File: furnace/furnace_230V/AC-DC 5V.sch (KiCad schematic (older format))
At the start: 14 parts

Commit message: Add files via upload
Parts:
- L?: value L_Core_Iron_Coupled_1243 -> PLA10AN3630R3D2
- PS?: value AC-DC 5V 700mA -> WX-DC12003 5V 0,7A
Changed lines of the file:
@@
 P 5900 4100
 F 0 "PS?" H 5900 4425 50  0000 C CNN
-F 1 "AC-DC 5V 700mA" H 5900 4334 50  0000 C CNN
+F 1 "WX-DC12003 5V 0,7A" H 5900 4334 50  0000 C CNN
 F 2 "" H 5900 3800 50  0001 C CNN
 F 3 "" H 6300 3750 50  0001 C CNN
@@
 P 4050 4100
 F 0 "L?" H 4050 4381 50  0000 C CNN
-F 1 "L_Core_Iron_Coupled_1243" H 4050 4290 50  0000 C CNN
+F 1 "PLA10AN3630R3D2" H 4050 4290 50  0000 C CNN
 F 2 "" H 4050 4100 50  0001 C CNN
 F 3 "~" H 4050 4100 50  0001 C CNN

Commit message: Add files via upload
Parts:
- C1, C2: renamed from C?; footprint (none) -> Capacitor_THT:C_Rect_L18.0mm_W7.0mm_P15.00mm_FKS3_FKP3; symbol Device:C -> furnace_230V-rescue:C-Device
- C3, C4: renamed from C?; footprint (none) -> Capacitor_SMD:C_1206_3216Metric_Pad1.33x1.80mm_HandSolder; symbol Device:C -> furnace_230V-rescue:C-Device
- C5: renamed from C?; footprint (none) -> Capacitor_SMD:C_Elec_5x5.4; symbol Device:CP -> furnace_230V-rescue:CP-Device
- D1: renamed from D?; footprint (none) -> Diode_SMD:D_SMA-SMB_Universal_Handsoldering; symbol Device:D_TVS -> furnace_230V-rescue:D_TVS-Device
- D2: renamed from D?; footprint (none) -> LED_SMD:LED_1206_3216Metric_Pad1.42x1.75mm_HandSolder; symbol Device:LED -> furnace_230V-rescue:LED-Device
- F1: renamed from F?; footprint (none) -> Fuse:Fuseholder_Cylinder-5x20mm_Stelvio-Kontek_PTF78_Horizontal_Open; symbol Device:Fuse -> furnace_230V-rescue:Fuse-Device
- L1: renamed from L?; symbol Device:L_Core_Iron_Coupled_1243 -> furnace_230V-rescue:L_Core_Iron_Coupled_1243-Device
- L2: renamed from L?; symbol Device:L -> furnace_230V-rescue:L-Device
- R1: renamed from R?; symbol Device:R -> furnace_230V-rescue:R-Device
- TP1, TP2: renamed from TP?; symbol Connector:TestPoint -> furnace_230V-rescue:TestPoint-Connector
- gave numbers to parts that had none: 1
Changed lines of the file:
@@
 $EndDescr
 $Comp
-L ac-dc:AC-DC PS?
+L ac-dc:AC-DC PS1
 U 1 1 60AB52E3
 P 5900 4100
-F 0 "PS?" H 5900 4425 50  0000 C CNN
+F 0 "PS1" H 5900 4425 50  0000 C CNN
 F 1 "WX-DC12003 5V 0,7A" H 5900 4334 50  0000 C CNN
 F 2 "" H 5900 3800 50  0001 C CNN
@@
 $EndComp
 $Comp
-L Device:C C?
+L furnace_230V-rescue:C-Device C1
 U 1 1 60ABB472
 P 3000 4150
-F 0 "C?" H 3115 4196 50  0000 L CNN
+F 0 "C1" H 3115 4196 50  0000 L CNN
 F 1 "0,15 275V" H 3115 4105 50  0000 L CNN
-F 2 "" H 3038 4000 50  0001 C CNN
+F 2 "Capacitor_THT:C_Rect_L18.0mm_W7.0mm_P15.00mm_FKS3_FKP3" H 3038 4000 50  0001 C CNN
 F 3 "~" H 3000 4150 50  0001 C CNN
 	1    3000 4150
@@
 $EndComp
 $Comp
-L Device:C C?
+L furnace_230V-rescue:C-Device C2
 U 1 1 60ABBB35
 P 4750 4150
-F 0 "C?" H 4865 4196 50  0000 L CNN
+F 0 "C2" H 4865 4196 50  0000 L CNN
 F 1 "0,15 275V" H 4865 4105 50  0000 L CNN
-F 2 "" H 4788 4000 50  0001 C CNN
+F 2 "Capacitor_THT:C_Rect_L18.0mm_W7.0mm_P15.00mm_FKS3_FKP3" H 4788 4000 50  0001 C CNN
 F 3 "~" H 4750 4150 50  0001 C CNN
 	1    4750 4150
@@
 $EndComp
 $Comp
-L Device:L_Core_Iron_Coupled_1243 L?
+L furnace_230V-rescue:L_Core_Iron_Coupled_1243-Device L1
 U 1 1 60ABCAA3
 P 4050 4100
-F 0 "L?" H 4050 4381 50  0000 C CNN
+F 0 "L1" H 4050 4381 50  0000 C CNN
 F 1 "PLA10AN3630R3D2" H 4050 4290 50  0000 C CNN
 F 2 "" H 4050 4100 50  0001 C CNN
@@
 $EndComp
 $Comp
-L Device:C C?
+L furnace_230V-rescue:C-Device C3
 U 1 1 60ABD84E
 P 6750 4150
-F 0 "C?" H 6865 4196 50  0000 L CNN
+F 0 "C3" H 6865 4196 50  0000 L CNN
 F 1 "10u" H 6865 4105 50  0000 L CNN
-F 2 "" H 6788 4000 50  0001 C CNN
+F 2 "Capacitor_SMD:C_1206_3216Metric_Pad1.33x1.80mm_HandSolder" H 6788 4000 50  0001 C CNN
 F 3 "~" H 6750 4150 50  0001 C CNN
 	1    6750 4150
@@
 $EndComp
 $Comp
-L Device:C C?
+L furnace_230V-rescue:C-Device C4
 U 1 1 60ABDA72
 P 7500 4150
-F 0 "C?" H 7615 4196 50  0000 L CNN
+F 0 "C4" H 7615 4196 50  0000 L CNN
 F 1 "10u" H 7615 4105 50  0000 L CNN
-F 2 "" H 7538 4000 50  0001 C CNN
+F 2 "Capacitor_SMD:C_1206_3216Metric_Pad1.33x1.80mm_HandSolder" H 7538 4000 50  0001 C CNN
 F 3 "~" H 7500 4150 50  0001 C CNN
 	1    7500 4150
@@
 $EndComp
 $Comp
-L Device:L L?
+L furnace_230V-rescue:L-Device L2
 U 1 1 60ABDC2D
 P 7250 4000
-F 0 "L?" V 7350 4000 50  0000 C CNN
+F 0 "L2" V 7350 4000 50  0000 C CNN
 F 1 "L" V 7200 4000 50  0000 C CNN
 F 2 "" H 7250 4000 50  0001 C CNN
@@
 $EndComp
 $Comp
-L Device:D_TVS D?
+L furnace_230V-rescue:D_TVS-Device D1
 U 1 1 60ABE587
 P 8000 4150
-F 0 "D?" V 7954 4230 50  0000 L CNN
+F 0 "D1" V 7954 4230 50  0000 L CNN
 F 1 "D_TVS" V 8045 4230 50  0000 L CNN
-F 2 "" H 8000 4150 50  0001 C CNN
+F 2 "Diode_SMD:D_SMA-SMB_Universal_Handsoldering" H 8000 4150 50  0001 C CNN
 F 3 "~" H 8000 4150 50  0001 C CNN
 	1    8000 4150
@@
 $EndComp
 $Comp
-L Device:Fuse F?
+L furnace_230V-rescue:Fuse-Device F1
 U 1 1 60ABEDE5
 P 2350 4000
-F 0 "F?" V 2250 4000 50  0000 C CNN
+F 0 "F1" V 2250 4000 50  0000 C CNN
 F 1 "0,1A" V 2450 4000 50  0000 C CNN
-F 2 "" V 2280 4000 50  0001 C CNN
+F 2 "Fuse:Fuseholder_Cylinder-5x20mm_Stelvio-Kontek_PTF78_Horizontal_Open" V 2280 4000 50  0001 C CNN
 F 3 "~" H 2350 4000 50  0001 C CNN
 	1    2350 4000
@@
 $EndComp
 $Comp
-L Connector:TestPoint TP?
+L furnace_230V-rescue:TestPoint-Connector TP?
 U 1 1 60ACEC46
 P 7000 4000
@@
 AR Path="/609CA6A8/60AE5653/60ACEC46" Ref="TP?"  Part="1"
 AR Path="/60AAC605/60ACEC46" Ref="TP?"  Part="1"
-AR Path="/60AABABA/60ACEC46" Ref="TP?"  Part="1"
-F 0 "TP?" H 7058 4118 50  0000 L CNN
+AR Path="/60AABABA/60ACEC46" Ref="TP1"  Part="1"
+F 0 "TP1" H 7058 4118 50  0000 L CNN
 F 1 "TestPoint" H 7058 4027 50  0001 L CNN
 F 2 "" H 7200 4000 50  0001 C CNN
@@
 $EndComp
 $Comp
-L Connector:TestPoint TP?
+L furnace_230V-rescue:TestPoint-Connector TP?
 U 1 1 60ACED6E
 P 8750 4000
@@
 AR Path="/609CA6A8/60AE5653/60ACED6E" Ref="TP?"  Part="1"
 AR Path="/60AAC605/60ACED6E" Ref="TP?"  Part="1"
-AR Path="/60AABABA/60ACED6E" Ref="TP?"  Part="1"
-F 0 "TP?" H 8808 4118 50  0000 L CNN
+AR Path="/60AABABA/60ACED6E" Ref="TP2"  Part="1"
+F 0 "TP2" H 8808 4118 50  0000 L CNN
 F 1 "TestPoint" H 8808 4027 50  0001 L CNN
 F 2 "" H 8950 4000 50  0001 C CNN
@@
 $EndComp
 $Comp
-L Device:R R?
+L furnace_230V-rescue:R-Device R?
 U 1 1 60AD2417
 P 9000 4150
@@
 AR Path="/60AAC605/60AD2417" Ref="R?"  Part="1"
 AR Path="/60AAE212/60AD2417" Ref="R?"  Part="1"
-AR Path="/60AABABA/60AD2417" Ref="R?"  Part="1"
-F 0 "R?" H 9070 4196 50  0000 L CNN
+AR Path="/60AABABA/60AD2417" Ref="R1"  Part="1"
+F 0 "R1" H 9070 4196 50  0000 L CNN
 F 1 "680" H 9070 4105 50  0000 L CNN
 F 2 "Resistor_SMD:R_0603_1608Metric_Pad0.98x0.95mm_HandSolder" V 8930 4150 50  0001 C CNN
@@
 $EndComp
 $Comp
-L Device:LED D?
+L furnace_230V-rescue:LED-Device D2
 U 1 1 60AD2617
 P 9000 4650
-F 0 "D?" V 9039 4532 50  0000 R CNN
+F 0 "D2" V 9039 4532 50  0000 R CNN
 F 1 "LED" V 8948 4532 50  0000 R CNN
-F 2 "" H 9000 4650 50  0001 C CNN
+F 2 "LED_SMD:LED_1206_3216Metric_Pad1.42x1.75mm_HandSolder" H 9000 4650 50  0001 C CNN
 F 3 "~" H 9000 4650 50  0001 C CNN
 	1    9000 4650
@@
 	7500 4000 8000 4000
 $Comp
-L Device:CP C?
+L furnace_230V-rescue:CP-Device C5
 U 1 1 60B2B0B1
 P 8500 4150
-F 0 "C?" H 8618 4196 50  0000 L CNN
+F 0 "C5" H 8618 4196 50  0000 L CNN
 F 1 "47u" H 8618 4105 50  0000 L CNN
-F 2 "" H 8538 4000 50  0001 C CNN
+F 2 "Capacitor_SMD:C_Elec_5x5.4" H 8538 4000 50  0001 C CNN
 F 3 "~" H 8500 4150 50  0001 C CNN
 	1    8500 4150

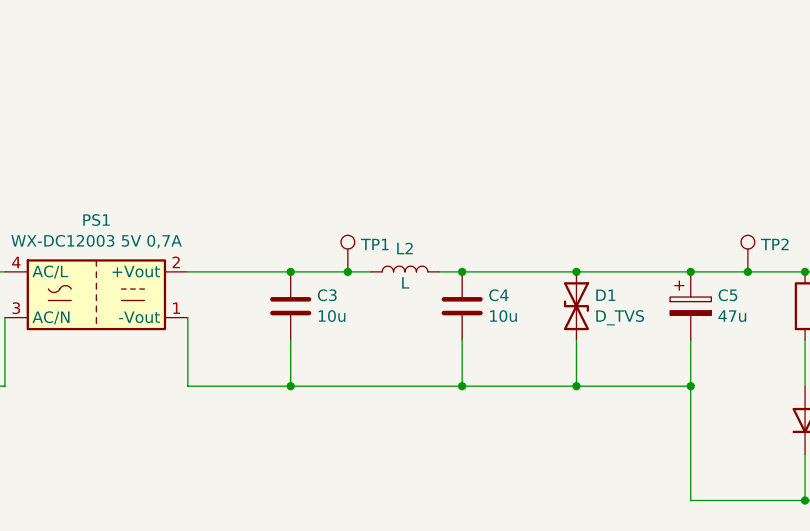
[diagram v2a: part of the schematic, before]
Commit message: Add files via upload
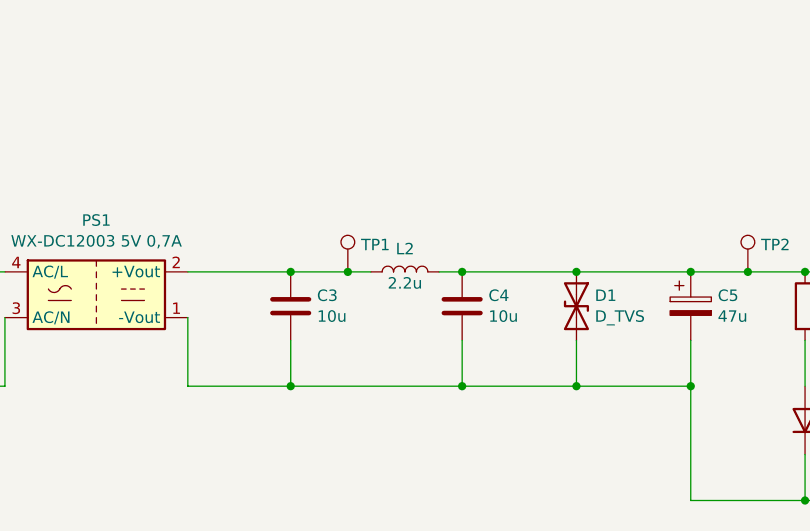
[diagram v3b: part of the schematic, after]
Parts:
- L2: value L -> 2.2u; footprint (none) -> Inductor_SMD:L_12x12mm_H8mm
- TP1, TP2: footprint (none) -> MountingHole:MountingHole_2.2mm_M2_DIN965_Pad_TopBottom
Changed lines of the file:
@@
 P 7250 4000
 F 0 "L2" V 7350 4000 50  0000 C CNN
-F 1 "L" V 7200 4000 50  0000 C CNN
-F 2 "" H 7250 4000 50  0001 C CNN
+F 1 "2.2u" V 7200 4000 50  0000 C CNN
+F 2 "Inductor_SMD:L_12x12mm_H8mm" H 7250 4000 50  0001 C CNN
 F 3 "~" H 7250 4000 50  0001 C CNN
 	1    7250 4000
@@
 F 0 "TP1" H 7058 4118 50  0000 L CNN
 F 1 "TestPoint" H 7058 4027 50  0001 L CNN
-F 2 "" H 7200 4000 50  0001 C CNN
+F 2 "MountingHole:MountingHole_2.2mm_M2_DIN965_Pad_TopBottom" H 7200 4000 50  0001 C CNN
 F 3 "~" H 7200 4000 50  0001 C CNN
 	1    7000 4000
@@
 F 0 "TP2" H 8808 4118 50  0000 L CNN
 F 1 "TestPoint" H 8808 4027 50  0001 L CNN
-F 2 "" H 8950 4000 50  0001 C CNN
+F 2 "MountingHole:MountingHole_2.2mm_M2_DIN965_Pad_TopBottom" H 8950 4000 50  0001 C CNN
 F 3 "~" H 8950 4000 50  0001 C CNN
 	1    8750 4000

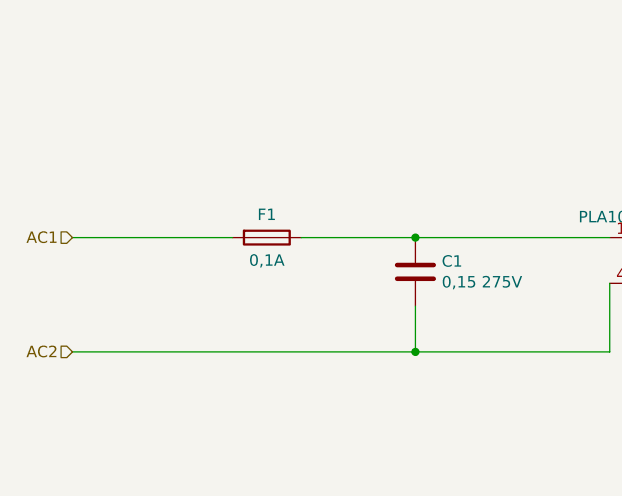
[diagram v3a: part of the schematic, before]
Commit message: Add files via upload
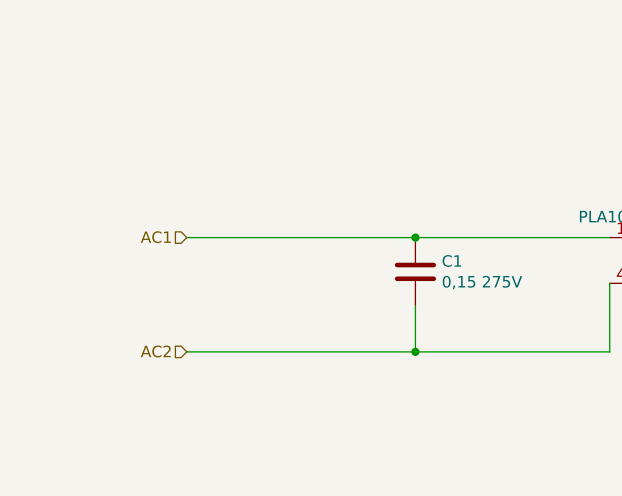
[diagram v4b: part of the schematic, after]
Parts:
- removed F1: 0,1A, Fuse:Fuseholder_Cylinder-5x20mm_Stelvio-Kontek_PTF78_Horizontal_Open, symbol furnace_230V-rescue:Fuse-Device
- C3, C4: footprint Capacitor_SMD:C_1206_3216Metric_Pad1.33x1.80mm_HandSolder -> Capacitor_SMD:C_1206_3216Metric_Pad1.42x1.75mm_HandSolder
- C5: footprint Capacitor_SMD:C_Elec_5x5.4 -> Capacitor_THT:CP_Radial_D5.0mm_P2.00mm
- D1: footprint Diode_SMD:D_SMA-SMB_Universal_Handsoldering -> Diode_SMD:D_SMB_Handsoldering
- D2: footprint LED_SMD:LED_1206_3216Metric_Pad1.42x1.75mm_HandSolder -> LED_SMD:LED_1206_3216Metric_ReverseMount_Hole1.8x2.4mm
- L1: footprint (none) -> furnace_230V:L_CommonMode_PLA10
- L2: footprint Inductor_SMD:L_12x12mm_H8mm -> Inductor_THT:L_Axial_L7.0mm_D3.3mm_P10.16mm_Horizontal_Fastron_MICC
- PS1: footprint (none) -> furnace_230V:WX-DC12003
- R1: footprint Resistor_SMD:R_0603_1608Metric_Pad0.98x0.95mm_HandSolder -> Resistor_SMD:R_0603_1608Metric_Pad1.05x0.95mm_HandSolder
- TP1, TP2: footprint MountingHole:MountingHole_2.2mm_M2_DIN965_Pad_TopBottom -> furnace_230V:TP
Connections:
- net AC1: now also C1.1, L1.1
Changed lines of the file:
@@
 F 0 "PS1" H 5900 4425 50  0000 C CNN
 F 1 "WX-DC12003 5V 0,7A" H 5900 4334 50  0000 C CNN
-F 2 "" H 5900 3800 50  0001 C CNN
+F 2 "furnace_230V:WX-DC12003" H 5900 3800 50  0001 C CNN
 F 3 "" H 6300 3750 50  0001 C CNN
 	1    5900 4100
@@
 F 0 "L1" H 4050 4381 50  0000 C CNN
 F 1 "PLA10AN3630R3D2" H 4050 4290 50  0000 C CNN
-F 2 "" H 4050 4100 50  0001 C CNN
+F 2 "furnace_230V:L_CommonMode_PLA10" H 4050 4100 50  0001 C CNN
 F 3 "~" H 4050 4100 50  0001 C CNN
 	1    4050 4100
@@
 F 0 "C3" H 6865 4196 50  0000 L CNN
 F 1 "10u" H 6865 4105 50  0000 L CNN
-F 2 "Capacitor_SMD:C_1206_3216Metric_Pad1.33x1.80mm_HandSolder" H 6788 4000 50  0001 C CNN
+F 2 "Capacitor_SMD:C_1206_3216Metric_Pad1.42x1.75mm_HandSolder" H 6788 4000 50  0001 C CNN
 F 3 "~" H 6750 4150 50  0001 C CNN
 	1    6750 4150
@@
 F 0 "C4" H 7615 4196 50  0000 L CNN
 F 1 "10u" H 7615 4105 50  0000 L CNN
-F 2 "Capacitor_SMD:C_1206_3216Metric_Pad1.33x1.80mm_HandSolder" H 7538 4000 50  0001 C CNN
+F 2 "Capacitor_SMD:C_1206_3216Metric_Pad1.42x1.75mm_HandSolder" H 7538 4000 50  0001 C CNN
 F 3 "~" H 7500 4150 50  0001 C CNN
 	1    7500 4150
@@
 F 0 "L2" V 7350 4000 50  0000 C CNN
 F 1 "2.2u" V 7200 4000 50  0000 C CNN
-F 2 "Inductor_SMD:L_12x12mm_H8mm" H 7250 4000 50  0001 C CNN
+F 2 "Inductor_THT:L_Axial_L7.0mm_D3.3mm_P10.16mm_Horizontal_Fastron_MICC" H 7250 4000 50  0001 C CNN
 F 3 "~" H 7250 4000 50  0001 C CNN
 	1    7250 4000
@@
 F 0 "D1" V 7954 4230 50  0000 L CNN
 F 1 "D_TVS" V 8045 4230 50  0000 L CNN
-F 2 "Diode_SMD:D_SMA-SMB_Universal_Handsoldering" H 8000 4150 50  0001 C CNN
+F 2 "Diode_SMD:D_SMB_Handsoldering" H 8000 4150 50  0001 C CNN
 F 3 "~" H 8000 4150 50  0001 C CNN
 	1    8000 4150
-	0    1    1    0
-$EndComp
-$Comp
-L furnace_230V-rescue:Fuse-Device F1
-U 1 1 60ABEDE5
-P 2350 4000
-F 0 "F1" V 2250 4000 50  0000 C CNN
-F 1 "0,1A" V 2450 4000 50  0000 C CNN
-F 2 "Fuse:Fuseholder_Cylinder-5x20mm_Stelvio-Kontek_PTF78_Horizontal_Open" V 2280 4000 50  0001 C CNN
-F 3 "~" H 2350 4000 50  0001 C CNN
-	1    2350 4000
 	0    1    1    0
 $EndComp
@@
 F 0 "TP1" H 7058 4118 50  0000 L CNN
 F 1 "TestPoint" H 7058 4027 50  0001 L CNN
-F 2 "MountingHole:MountingHole_2.2mm_M2_DIN965_Pad_TopBottom" H 7200 4000 50  0001 C CNN
+F 2 "furnace_230V:TP" H 7200 4000 50  0001 C CNN
 F 3 "~" H 7200 4000 50  0001 C CNN
 	1    7000 4000
@@
 F 0 "TP2" H 8808 4118 50  0000 L CNN
 F 1 "TestPoint" H 8808 4027 50  0001 L CNN
-F 2 "MountingHole:MountingHole_2.2mm_M2_DIN965_Pad_TopBottom" H 8950 4000 50  0001 C CNN
+F 2 "furnace_230V:TP" H 8950 4000 50  0001 C CNN
 F 3 "~" H 8950 4000 50  0001 C CNN
 	1    8750 4000
@@
 F 0 "R1" H 9070 4196 50  0000 L CNN
 F 1 "680" H 9070 4105 50  0000 L CNN
-F 2 "Resistor_SMD:R_0603_1608Metric_Pad0.98x0.95mm_HandSolder" V 8930 4150 50  0001 C CNN
+F 2 "Resistor_SMD:R_0603_1608Metric_Pad1.05x0.95mm_HandSolder" V 8930 4150 50  0001 C CNN
 F 3 "~" H 9000 4150 50  0001 C CNN
 	1    9000 4150
@@
 F 0 "D2" V 9039 4532 50  0000 R CNN
 F 1 "LED" V 8948 4532 50  0000 R CNN
-F 2 "LED_SMD:LED_1206_3216Metric_Pad1.42x1.75mm_HandSolder" H 9000 4650 50  0001 C CNN
+F 2 "LED_SMD:LED_1206_3216Metric_ReverseMount_Hole1.8x2.4mm" H 9000 4650 50  0001 C CNN
 F 3 "~" H 9000 4650 50  0001 C CNN
 	1    9000 4650
@@
 Text HLabel 10000 5000 2    50   Output ~ 0
 GND
-Text HLabel 1500 4000 0    50   Input ~ 0
+Text HLabel 2000 4000 0    50   Input ~ 0
 AC1
-Text HLabel 1500 4500 0    50   Input ~ 0
+Text HLabel 2000 4500 0    50   Input ~ 0
 AC2
 Wire Wire Line
-	1500 4000 2200 4000
-Wire Wire Line
-	2500 4000 3000 4000
+	2000 4000 3000 4000
 Wire Wire Line
 	3000 4000 3850 4000
@@
 Connection ~ 4750 4000
 Wire Wire Line
-	1500 4500 3000 4500
+	2000 4500 3000 4500
 Wire Wire Line
 	3850 4500 3850 4200
@@
 F 0 "C5" H 8618 4196 50  0000 L CNN
 F 1 "47u" H 8618 4105 50  0000 L CNN
-F 2 "Capacitor_SMD:C_Elec_5x5.4" H 8538 4000 50  0001 C CNN
+F 2 "Capacitor_THT:CP_Radial_D5.0mm_P2.00mm" H 8538 4000 50  0001 C CNN
 F 3 "~" H 8500 4150 50  0001 C CNN
 	1    8500 4150

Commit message: Add files via upload
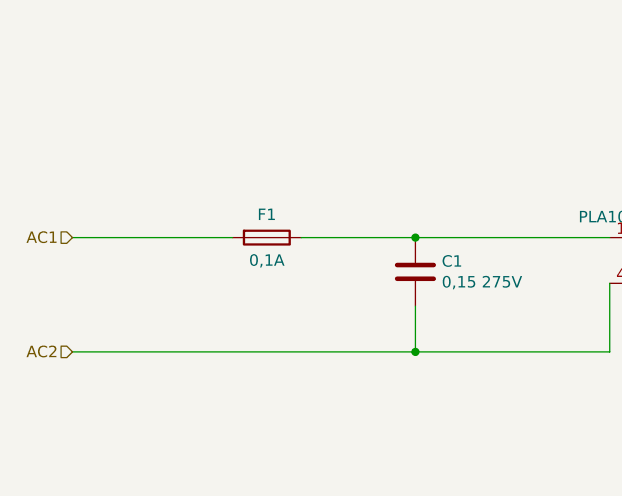
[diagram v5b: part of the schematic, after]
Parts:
- added F1: 0,1A, Fuse:Fuseholder_Cylinder-5x20mm_Stelvio-Kontek_PTF78_Horizontal_Open, symbol furnace_230V-rescue:Fuse-Device
- C3, C4: footprint Capacitor_SMD:C_1206_3216Metric_Pad1.42x1.75mm_HandSolder -> Capacitor_SMD:C_1206_3216Metric_Pad1.33x1.80mm_HandSolder
- C5: footprint Capacitor_THT:CP_Radial_D5.0mm_P2.00mm -> Capacitor_SMD:C_Elec_5x5.4
- D1: footprint Diode_SMD:D_SMB_Handsoldering -> Diode_SMD:D_SMA-SMB_Universal_Handsoldering
- D2: footprint LED_SMD:LED_1206_3216Metric_ReverseMount_Hole1.8x2.4mm -> LED_SMD:LED_1206_3216Metric_Pad1.42x1.75mm_HandSolder
- L1: footprint furnace_230V:L_CommonMode_PLA10 -> (none)
- L2: footprint Inductor_THT:L_Axial_L7.0mm_D3.3mm_P10.16mm_Horizontal_Fastron_MICC -> Inductor_SMD:L_12x12mm_H8mm
- PS1: footprint furnace_230V:WX-DC12003 -> (none)
- R1: footprint Resistor_SMD:R_0603_1608Metric_Pad1.05x0.95mm_HandSolder -> Resistor_SMD:R_0603_1608Metric_Pad0.98x0.95mm_HandSolder
- TP1, TP2: footprint furnace_230V:TP -> MountingHole:MountingHole_2.2mm_M2_DIN965_Pad_TopBottom
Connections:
- net AC1: now also F1.2; no longer C1.1, L1.1
- new net: C1.1, F1.1, L1.1
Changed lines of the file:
@@
 F 0 "PS1" H 5900 4425 50  0000 C CNN
 F 1 "WX-DC12003 5V 0,7A" H 5900 4334 50  0000 C CNN
-F 2 "furnace_230V:WX-DC12003" H 5900 3800 50  0001 C CNN
+F 2 "" H 5900 3800 50  0001 C CNN
 F 3 "" H 6300 3750 50  0001 C CNN
 	1    5900 4100
@@
 F 0 "L1" H 4050 4381 50  0000 C CNN
 F 1 "PLA10AN3630R3D2" H 4050 4290 50  0000 C CNN
-F 2 "furnace_230V:L_CommonMode_PLA10" H 4050 4100 50  0001 C CNN
+F 2 "" H 4050 4100 50  0001 C CNN
 F 3 "~" H 4050 4100 50  0001 C CNN
 	1    4050 4100
@@
 F 0 "C3" H 6865 4196 50  0000 L CNN
 F 1 "10u" H 6865 4105 50  0000 L CNN
-F 2 "Capacitor_SMD:C_1206_3216Metric_Pad1.42x1.75mm_HandSolder" H 6788 4000 50  0001 C CNN
+F 2 "Capacitor_SMD:C_1206_3216Metric_Pad1.33x1.80mm_HandSolder" H 6788 4000 50  0001 C CNN
 F 3 "~" H 6750 4150 50  0001 C CNN
 	1    6750 4150
@@
 F 0 "C4" H 7615 4196 50  0000 L CNN
 F 1 "10u" H 7615 4105 50  0000 L CNN
-F 2 "Capacitor_SMD:C_1206_3216Metric_Pad1.42x1.75mm_HandSolder" H 7538 4000 50  0001 C CNN
+F 2 "Capacitor_SMD:C_1206_3216Metric_Pad1.33x1.80mm_HandSolder" H 7538 4000 50  0001 C CNN
 F 3 "~" H 7500 4150 50  0001 C CNN
 	1    7500 4150
@@
 F 0 "L2" V 7350 4000 50  0000 C CNN
 F 1 "2.2u" V 7200 4000 50  0000 C CNN
-F 2 "Inductor_THT:L_Axial_L7.0mm_D3.3mm_P10.16mm_Horizontal_Fastron_MICC" H 7250 4000 50  0001 C CNN
+F 2 "Inductor_SMD:L_12x12mm_H8mm" H 7250 4000 50  0001 C CNN
 F 3 "~" H 7250 4000 50  0001 C CNN
 	1    7250 4000
@@
 F 0 "D1" V 7954 4230 50  0000 L CNN
 F 1 "D_TVS" V 8045 4230 50  0000 L CNN
-F 2 "Diode_SMD:D_SMB_Handsoldering" H 8000 4150 50  0001 C CNN
+F 2 "Diode_SMD:D_SMA-SMB_Universal_Handsoldering" H 8000 4150 50  0001 C CNN
 F 3 "~" H 8000 4150 50  0001 C CNN
 	1    8000 4150
+	0    1    1    0
+$EndComp
+$Comp
+L furnace_230V-rescue:Fuse-Device F1
+U 1 1 60ABEDE5
+P 2350 4000
+F 0 "F1" V 2250 4000 50  0000 C CNN
+F 1 "0,1A" V 2450 4000 50  0000 C CNN
+F 2 "Fuse:Fuseholder_Cylinder-5x20mm_Stelvio-Kontek_PTF78_Horizontal_Open" V 2280 4000 50  0001 C CNN
+F 3 "~" H 2350 4000 50  0001 C CNN
+	1    2350 4000
 	0    1    1    0
 $EndComp
@@
 F 0 "TP1" H 7058 4118 50  0000 L CNN
 F 1 "TestPoint" H 7058 4027 50  0001 L CNN
-F 2 "furnace_230V:TP" H 7200 4000 50  0001 C CNN
+F 2 "MountingHole:MountingHole_2.2mm_M2_DIN965_Pad_TopBottom" H 7200 4000 50  0001 C CNN
 F 3 "~" H 7200 4000 50  0001 C CNN
 	1    7000 4000
@@
 F 0 "TP2" H 8808 4118 50  0000 L CNN
 F 1 "TestPoint" H 8808 4027 50  0001 L CNN
-F 2 "furnace_230V:TP" H 8950 4000 50  0001 C CNN
+F 2 "MountingHole:MountingHole_2.2mm_M2_DIN965_Pad_TopBottom" H 8950 4000 50  0001 C CNN
 F 3 "~" H 8950 4000 50  0001 C CNN
 	1    8750 4000
@@
 F 0 "R1" H 9070 4196 50  0000 L CNN
 F 1 "680" H 9070 4105 50  0000 L CNN
-F 2 "Resistor_SMD:R_0603_1608Metric_Pad1.05x0.95mm_HandSolder" V 8930 4150 50  0001 C CNN
+F 2 "Resistor_SMD:R_0603_1608Metric_Pad0.98x0.95mm_HandSolder" V 8930 4150 50  0001 C CNN
 F 3 "~" H 9000 4150 50  0001 C CNN
 	1    9000 4150
@@
 F 0 "D2" V 9039 4532 50  0000 R CNN
 F 1 "LED" V 8948 4532 50  0000 R CNN
-F 2 "LED_SMD:LED_1206_3216Metric_ReverseMount_Hole1.8x2.4mm" H 9000 4650 50  0001 C CNN
+F 2 "LED_SMD:LED_1206_3216Metric_Pad1.42x1.75mm_HandSolder" H 9000 4650 50  0001 C CNN
 F 3 "~" H 9000 4650 50  0001 C CNN
 	1    9000 4650
@@
 Text HLabel 10000 5000 2    50   Output ~ 0
 GND
-Text HLabel 2000 4000 0    50   Input ~ 0
+Text HLabel 1500 4000 0    50   Input ~ 0
 AC1
-Text HLabel 2000 4500 0    50   Input ~ 0
+Text HLabel 1500 4500 0    50   Input ~ 0
 AC2
 Wire Wire Line
-	2000 4000 3000 4000
+	1500 4000 2200 4000
+Wire Wire Line
+	2500 4000 3000 4000
 Wire Wire Line
 	3000 4000 3850 4000
@@
 Connection ~ 4750 4000
 Wire Wire Line
-	2000 4500 3000 4500
+	1500 4500 3000 4500
 Wire Wire Line
 	3850 4500 3850 4200
@@
 F 0 "C5" H 8618 4196 50  0000 L CNN
 F 1 "47u" H 8618 4105 50  0000 L CNN
-F 2 "Capacitor_THT:CP_Radial_D5.0mm_P2.00mm" H 8538 4000 50  0001 C CNN
+F 2 "Capacitor_SMD:C_Elec_5x5.4" H 8538 4000 50  0001 C CNN
 F 3 "~" H 8500 4150 50  0001 C CNN
 	1    8500 4150
